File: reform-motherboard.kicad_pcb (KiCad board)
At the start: 4 copper layers, 130 x 100 mm, 188 parts, among them J1 TinyRex-J1-DF40C, J10 TEST_PMIC_ON, J11 TEST_ON, J12 USB_INT_3, J13 Conn_HDMI, J14 Conn_LVDS, J15 USB_INT_2, J16 Conn_LineIn, J17 Conn_LineOut, J18 TRRS, J19 Conn_BOOT, J2 TinyRex-J2-DF40C, J20 Conn_GPIO1, J21 Conn_GPIO2, J22 Conn_PWRON, J23 Conn_RESET, J24 Conn_01x04, J25 Conn_CONSOLE, J26 Conn_Backlight, J3 TinyRex-J3-DF40C, J4 693072010801, J5 USB_A, J6 Barrel_Jack, J7 USB_A, J8 TEST_3V, J9 USB_INT_1, P1 5622-4100-ML, P2 J0G-0003NL, Q1 2N7002, Q2 2N7002, Q3 2N7002, U1 MPCIE-Socket, U10 SGTL5000XNAA3, U11 TPS74801DRCR, U12 SN74LVC1G08DCKR, U13 TXB0104D, U14 CM2020-00TR, U2 MCP73123T-22SI/MF, U3 TPS61235RWLR, U4 AP1501A-33K5G-13, U5 SN74LVC1G14DBVR, U6 TPS74801DRCR, U7 INA260AIPW, U8 TUSB4041IPAPR, U9 TLV71311PDBV, Y1 24MHz

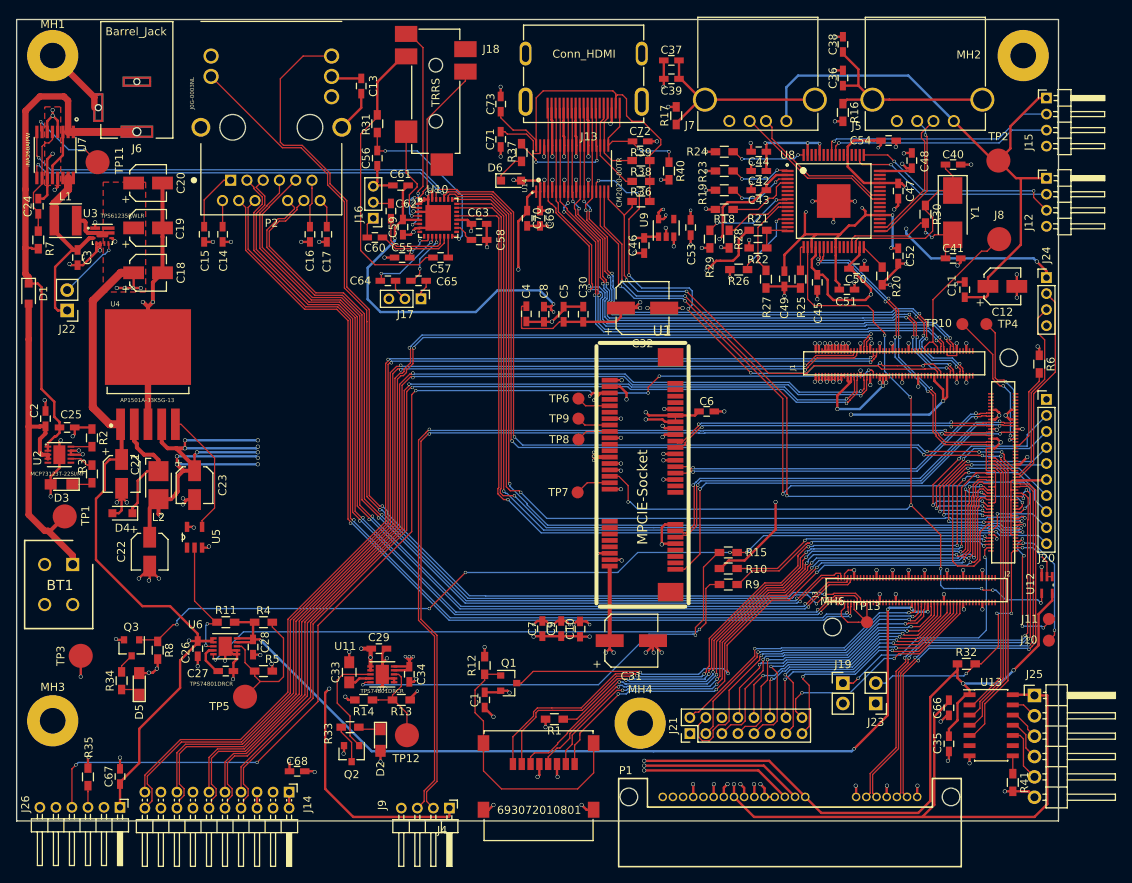
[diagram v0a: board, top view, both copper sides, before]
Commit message: manufacturing version 0.1
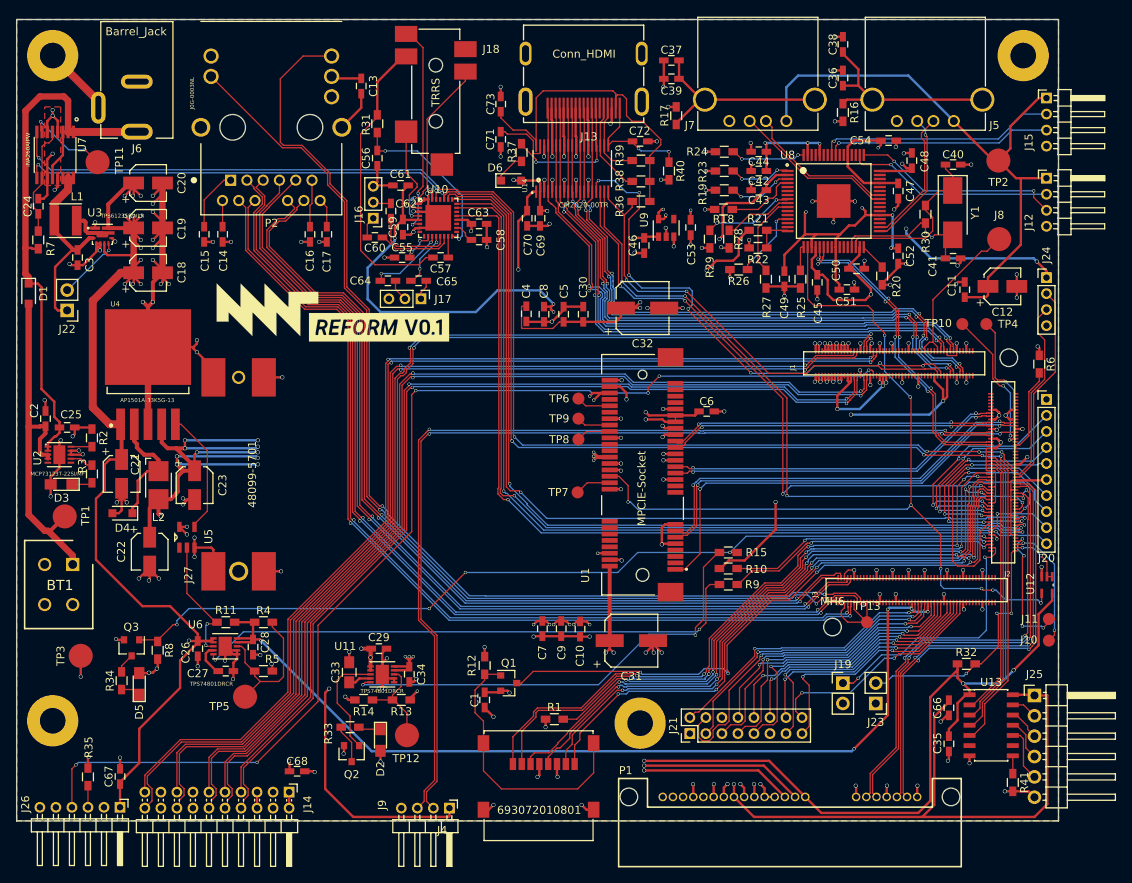
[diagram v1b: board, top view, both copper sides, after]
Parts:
- added G***: LOGO, mnt:mnt, F.Cu at (61.3, 56.2)
- added G***: LOGO, mnt:reform01, F.Cu at (75.2, 58.4)
- added J27: 48099-5701, 48099-5701:MOLEX_48099-5701, F.Cu at (57.7, 76.8)
- U1: footprint mpcie:mpcie-socket -> 67910-5700:MOLEX_67910-5700
- moved U1 10.7 mm to (108.1, 78.6)
- moved U5 0.95 mm to (51.2, 84.6)
- moved R18 0.10 mm to (118.2, 43.7)
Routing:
- net GND: track 421.2 -> 463.6 mm, vias 178 -> 191
- net +5V: track 346.0 -> 386.2 mm, vias 24 -> 33
- net HDMI_CEC_IN: track 67.5 -> 65.8 mm
- net +1V1: track 69.6 -> 68.3 mm, vias 12 -> 11
- net Net-(J19-Pad1): track 31.8 -> 32.8 mm
- net POK_3V3: track 112.3 -> 113.2 mm, vias 6 -> 5
- net Net-(J2-Pad29): track 28.8 -> 28.1 mm
- added copper zone on B.Cu, net GND
- removed copper zone on F.Cu, net +5V
